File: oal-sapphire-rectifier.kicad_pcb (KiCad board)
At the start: 2 copper layers, 100 x 80 mm, 18 parts, among them J1 LINE, J2 NEUTRAL, J3 GROUND, J4 OUTPUT, T1 TALEMA-25VA/12V, X1 MOUNTING_HOLE, X2 MOUNTING_HOLE, X3 MOUNTING_HOLE, X4 MOUNTING_HOLE

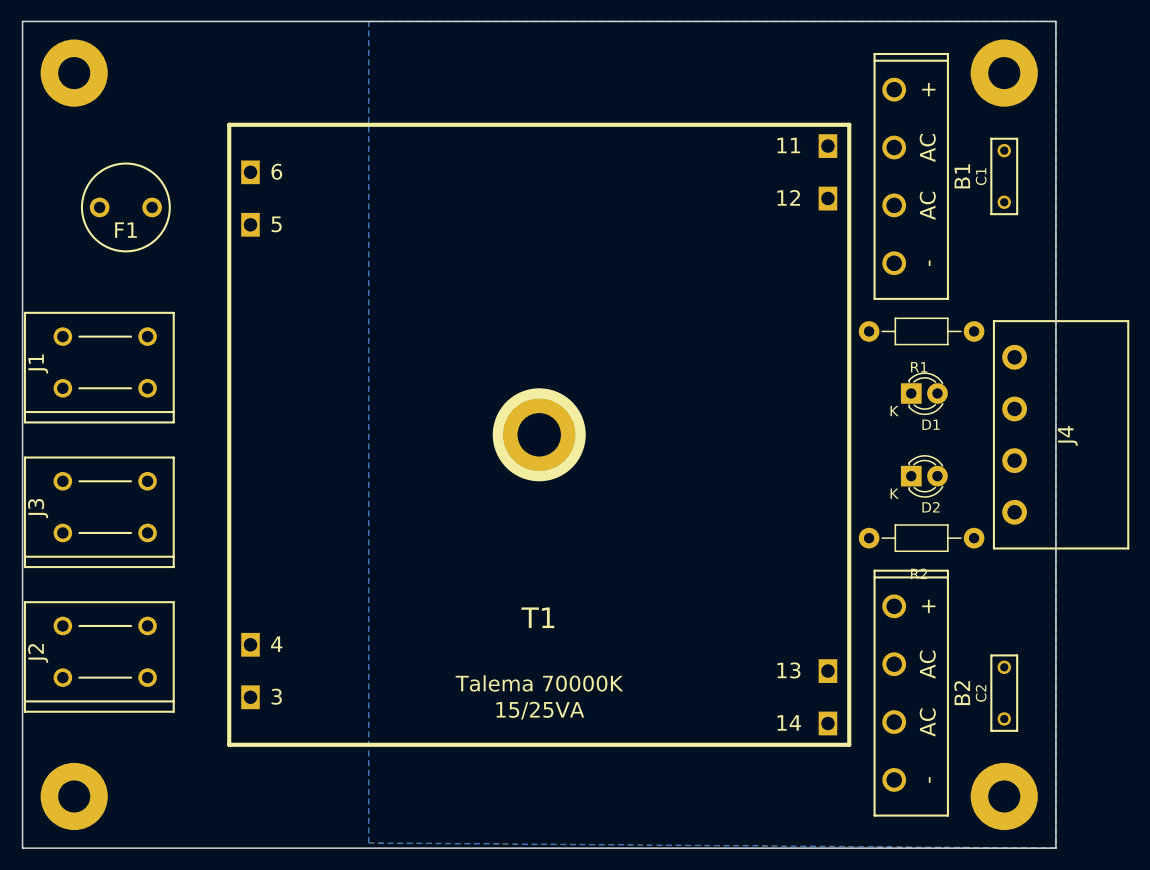
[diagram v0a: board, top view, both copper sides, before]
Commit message: initial layout
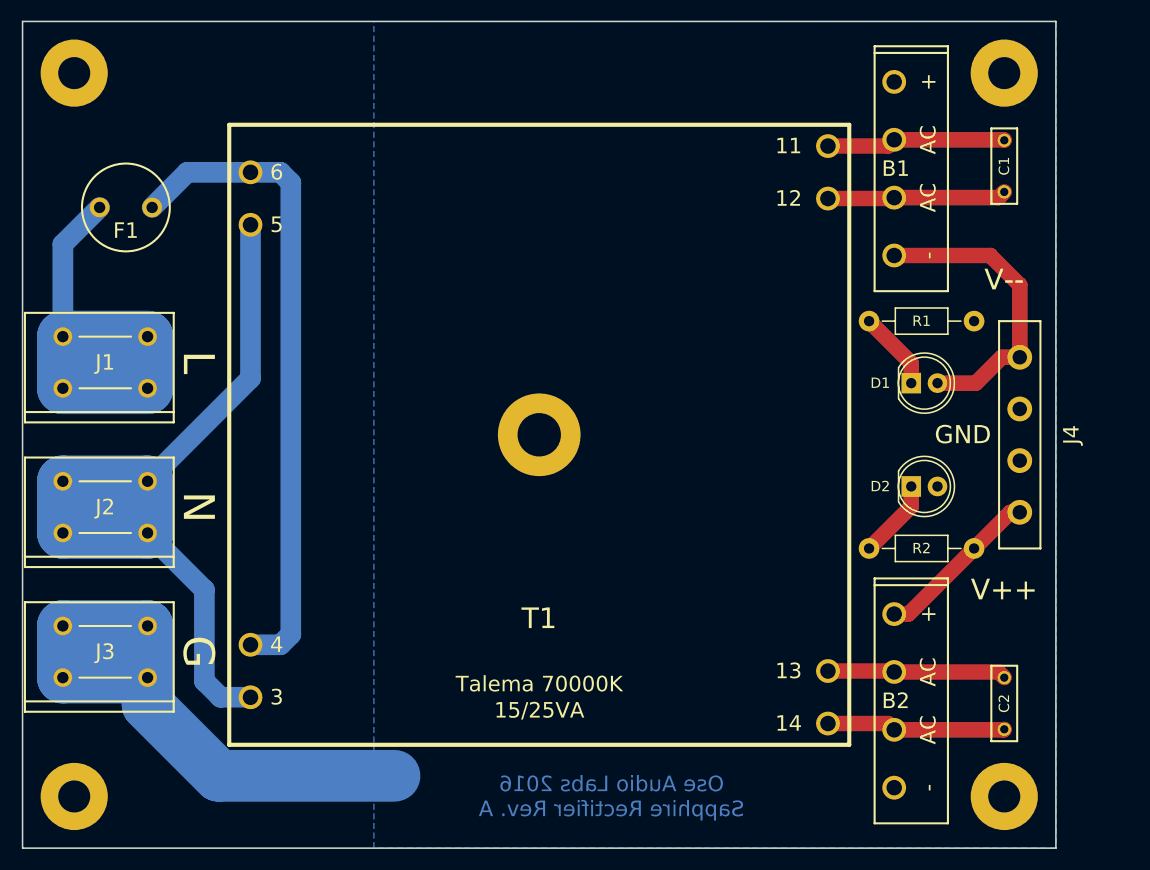
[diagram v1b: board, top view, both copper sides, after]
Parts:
- D1, D2: footprint LEDs:LED-3MM -> LEDs:LED-5MM
- J4: footprint ose-audio-labs:MSTBA-2.5_4-G -> MSTBA-2.5_4-G
- T1: footprint ose-audio-labs:TALEMA_70000K_15-25VA -> TALEMA_70000K_15-25VA
- moved J2 14.0 mm to (8.00, 7.00)
- moved J3 14.0 mm to (8.00, 21.0)
- moved C1 1.00 mm to (95.0, -26.0)
- moved C2 1.00 mm to (95.0, 26.0)
- moved D1 1.00 mm to (86.0, -5.00)
- moved D2 1.00 mm to (86.0, 5.00)
- moved R1 1.00 mm to (87.0, -11.0)
- moved R2 1.00 mm to (87.0, 11.0)
- moved B1 0.75 mm to (86.0, -25.8)
- moved B2 0.75 mm to (86.0, 25.8)
- moved J4 0.50 mm to (96.5, 0.00)
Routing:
- net 120V-NEUTRAL: track 0.00 -> 77.1 mm
- net Net-(F1-Pad2): track 0.00 -> 63.3 mm
- net GROUND: track 0.00 -> 56.0 mm
- net 120V-LINE: track 0.00 -> 40.4 mm
- net V++: track 0.00 -> 29.3 mm
- net Net-(B1-Pad3): track 0.00 -> 17.5 mm
- net Net-(B2-Pad2): track 0.00 -> 17.3 mm
- net Net-(B1-Pad2): track 0.00 -> 17.3 mm
- net Net-(B2-Pad3): track 0.00 -> 17.3 mm
- net V--: track 0.00 -> 16.2 mm
- net Net-(D2-Pad1): track 0.00 -> 7.69 mm
- net Net-(D1-Pad1): track 0.00 -> 7.69 mm
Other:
- net class Default: trace_width 1.2 -> 1.5
- net class MAINS: clearance 1.2 -> 2; trace_width 1.5 -> 2
- board text added: "G"
- board text added: "GND"
- board text added: "L"
- board text added: "N"
- board text added: "Ose Audio Labs 2016 Sapphire Rectifier Rev. A"
- board text added: "V++"
- board text added: "V--"
